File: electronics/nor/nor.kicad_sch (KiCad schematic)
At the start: 9 parts, among them Q1 NPN, Q2 NPN, Q3 NPN

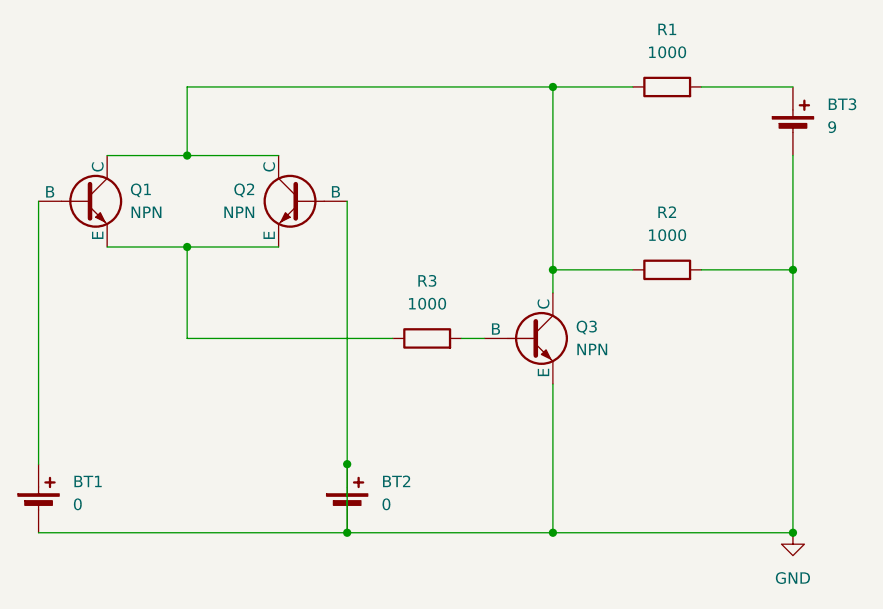
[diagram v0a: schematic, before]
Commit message: fix
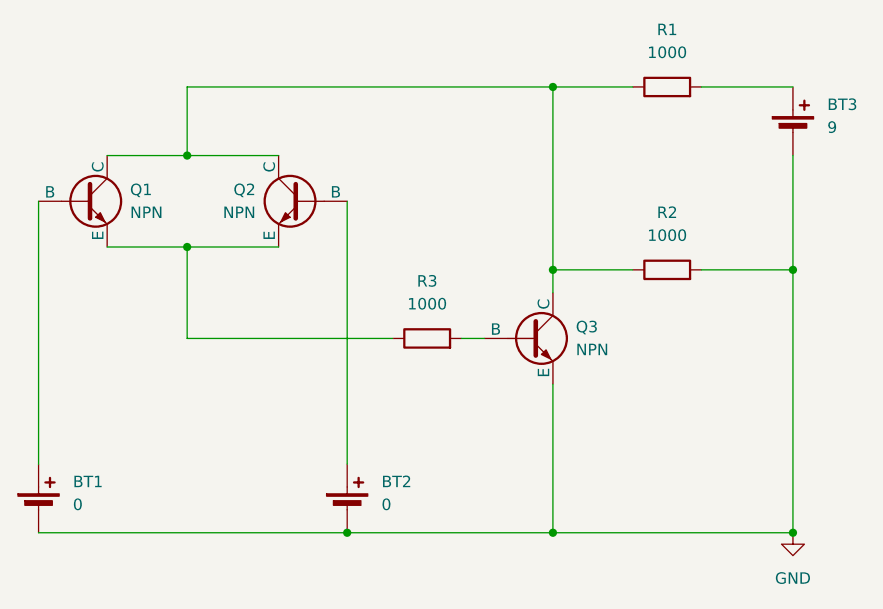
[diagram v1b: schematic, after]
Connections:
- net GND: no longer BT2.1 (+), Q2.2 (B)
- new net: BT2.1 (+), Q2.2 (B)
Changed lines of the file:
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@@
-	)
-	(junction
-		(at 90.17 85.09)
-		(diameter 0)
-		(color 0 0 0 0)
 	)
 	(junction
@@
 		(pts
 			(xy 139.7 63.5) (xy 139.7 92.71)
+		)
+		(stroke
+			(width 0)
+			(type default)
+		)
+	)
+	(wire
+		(pts
+			(xy 90.17 55.88) (xy 90.17 85.09)
 		)
 		(stroke
@@
 	(wire
 		(pts
-			(xy 90.17 85.09) (xy 90.17 92.71)
-		)
-		(stroke
-			(width 0)
-			(type default)
-		)
-	)
-	(wire
-		(pts
 			(xy 72.39 60.96) (xy 82.55 60.96)
 		)
 		(stroke
-			(width 0)
-			(type default)
-		)
-	)
-	(wire
-		(pts
-			(xy 90.17 55.88) (xy 90.17 85.09)
-		)
-		(stroke
